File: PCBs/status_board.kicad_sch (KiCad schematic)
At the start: 21 parts, among them J1 Conn_01x03, J2 Conn_01x03, J3 Conn_01x02, J4 Conn_01x04, J5 Conn_01x04, J6 Conn_01x04, J7 Conn_01x07, J8 Conn_01x07, J9 Conn_01x04

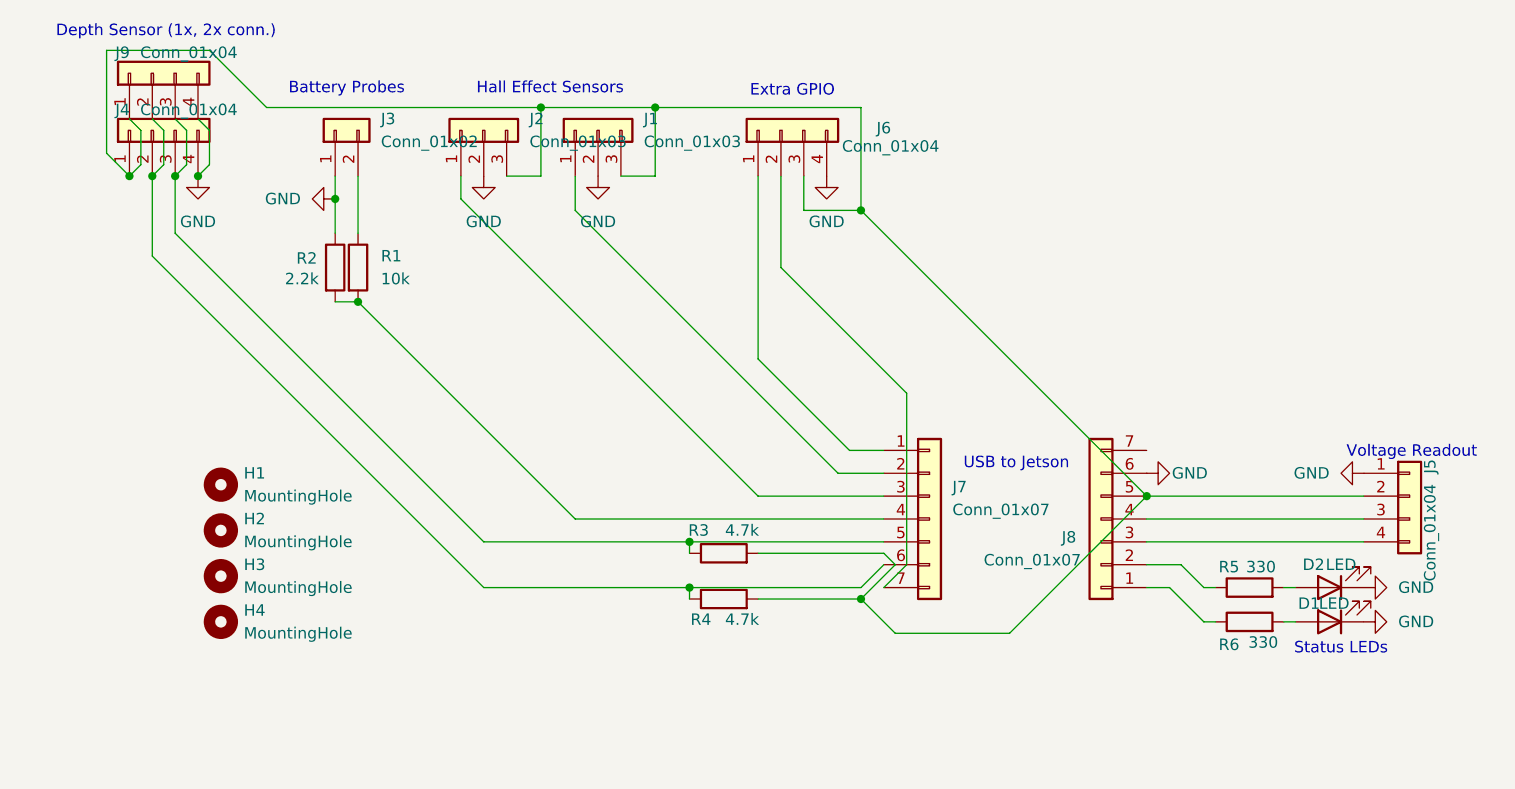
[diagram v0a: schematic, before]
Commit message: make sketch more compact
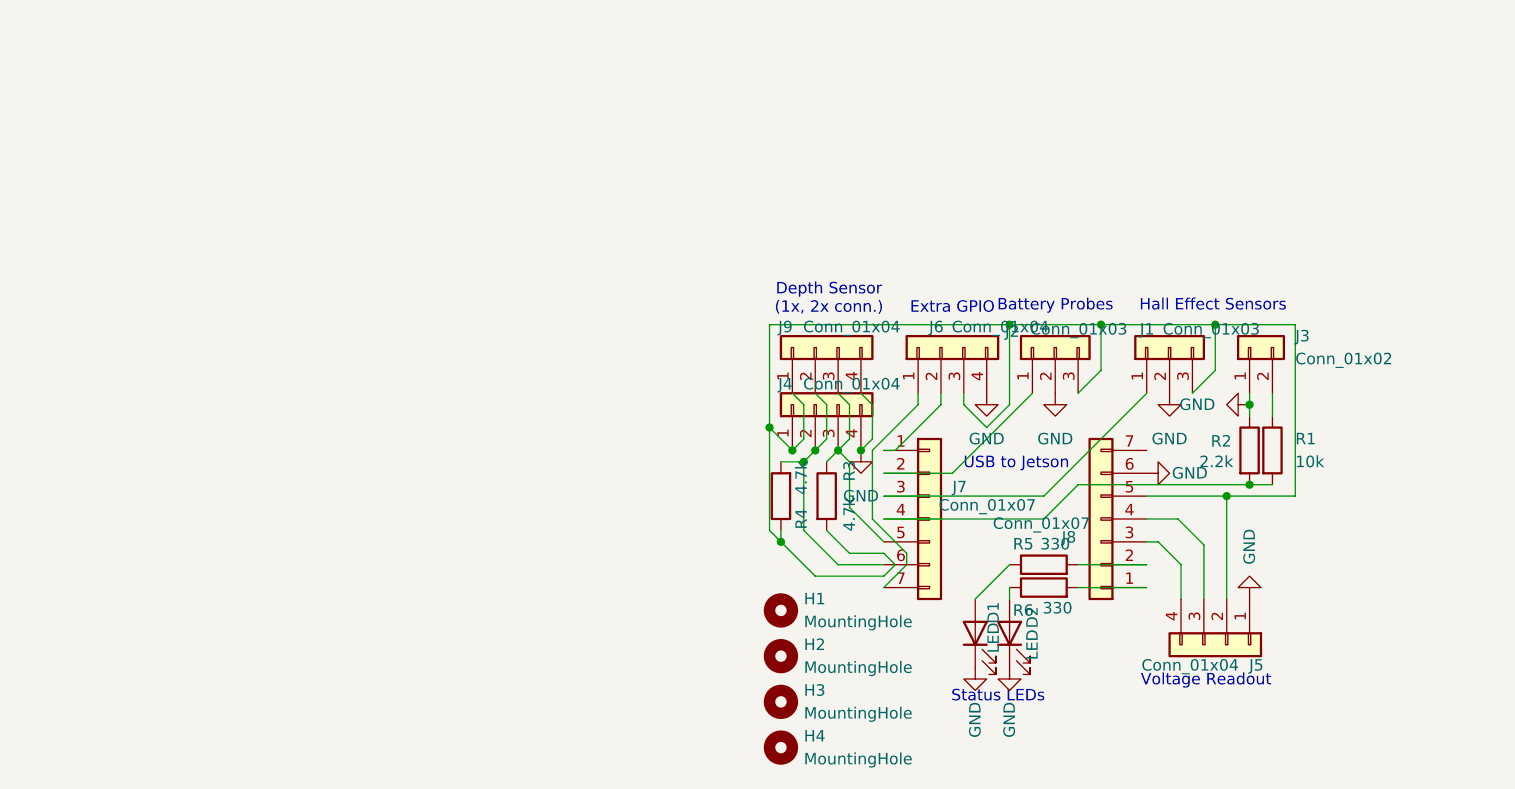
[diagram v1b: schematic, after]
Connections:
- net at R5.1: now also D2.2 (A); no longer J8.2 (Pin_2)
- net at R5.2: now also J8.2 (Pin_2); no longer D1.2 (A)
- net at J4.2 (Pin_2), J7.6 (Pin_6), J9.2 (Pin_2): now also R4.2; no longer R4.1
- net at J1.3 (Pin_3), J2.3 (Pin_3), J4.1 (Pin_1)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: now also R4.1; no longer R4.2
- net at J7.1 (Pin_1): now also J6.2 (Pin_2); no longer J6.1 (Pin_1)
- net at J7.2 (Pin_2): now also J2.1 (Pin_1); no longer J1.1 (Pin_1)
- net at J7.3 (Pin_3): now also J1.1 (Pin_1); no longer J2.1 (Pin_1)
- net at J7.7 (Pin_7): now also J6.1 (Pin_1); no longer J6.2 (Pin_2)
- net at R6.1: now also D1.2 (A); no longer J8.1 (Pin_1)
- net at R6.2: now also J8.1 (Pin_1); no longer D2.2 (A)
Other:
- moved on the sheet: D1, D2, H1, H2, H3, H4, J1, J2, J3, J4, J5, J6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

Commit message: first draft of board
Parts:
- J1, J2: footprint (none) -> Connector_JST:JST_GH_BM03B-GHS-TBT_1x03-1MP_P1.25mm_Vertical
- J5: footprint Connector_PinHeader_2.54mm:PinHeader_1x04_P2.54mm_Vertical -> Connector_PinSocket_2.54mm:PinSocket_1x04_P2.54mm_Vertical
- J6: footprint (none) -> Connector_JST:JST_GH_BM04B-GHS-TBT_1x04-1MP_P1.25mm_Vertical
- J7, J8: footprint Connector_PinHeader_2.54mm:PinHeader_1x07_P2.54mm_Vertical -> Connector_PinSocket_2.54mm:PinSocket_1x07_P2.54mm_Vertical
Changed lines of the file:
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@@
 			)
 		)
-		(property "Footprint" "Connector_PinHeader_2.54mm:PinHeader_1x07_P2.54mm_Vertical"
+		(property "Footprint" "Connector_PinSocket_2.54mm:PinSocket_1x07_P2.54mm_Vertical"
 			(at 135.89 102.87 0)
 			(hide yes)
@@
 			)
 		)
-		(property "Footprint" ""
+		(property "Footprint" "Connector_JST:JST_GH_BM03B-GHS-TBT_1x03-1MP_P1.25mm_Vertical"
 			(at 149.86 83.82 0)
 			(hide yes)
@@
 			)
 		)
-		(property "Footprint" "Connector_PinHeader_2.54mm:PinHeader_1x04_P2.54mm_Vertical"
+		(property "Footprint" "Connector_PinSocket_2.54mm:PinSocket_1x04_P2.54mm_Vertical"
 			(at 168.91 116.84 0)
 			(hide yes)
@@
 			)
 		)
-		(property "Footprint" ""
+		(property "Footprint" "Connector_JST:JST_GH_BM04B-GHS-TBT_1x04-1MP_P1.25mm_Vertical"
 			(at 137.16 83.82 0)
 			(hide yes)
@@
 			)
 		)
-		(property "Footprint" ""
+		(property "Footprint" "Connector_JST:JST_GH_BM03B-GHS-TBT_1x03-1MP_P1.25mm_Vertical"
 			(at 162.56 83.82 0)
 			(hide yes)
@@
 			)
 		)
-		(property "Footprint" "Connector_PinHeader_2.54mm:PinHeader_1x07_P2.54mm_Vertical"
+		(property "Footprint" "Connector_PinSocket_2.54mm:PinSocket_1x07_P2.54mm_Vertical"
 			(at 154.94 102.87 0)
 			(hide yes)
